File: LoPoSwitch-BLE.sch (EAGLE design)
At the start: 12 parts, among them Q1 2.5A/30V

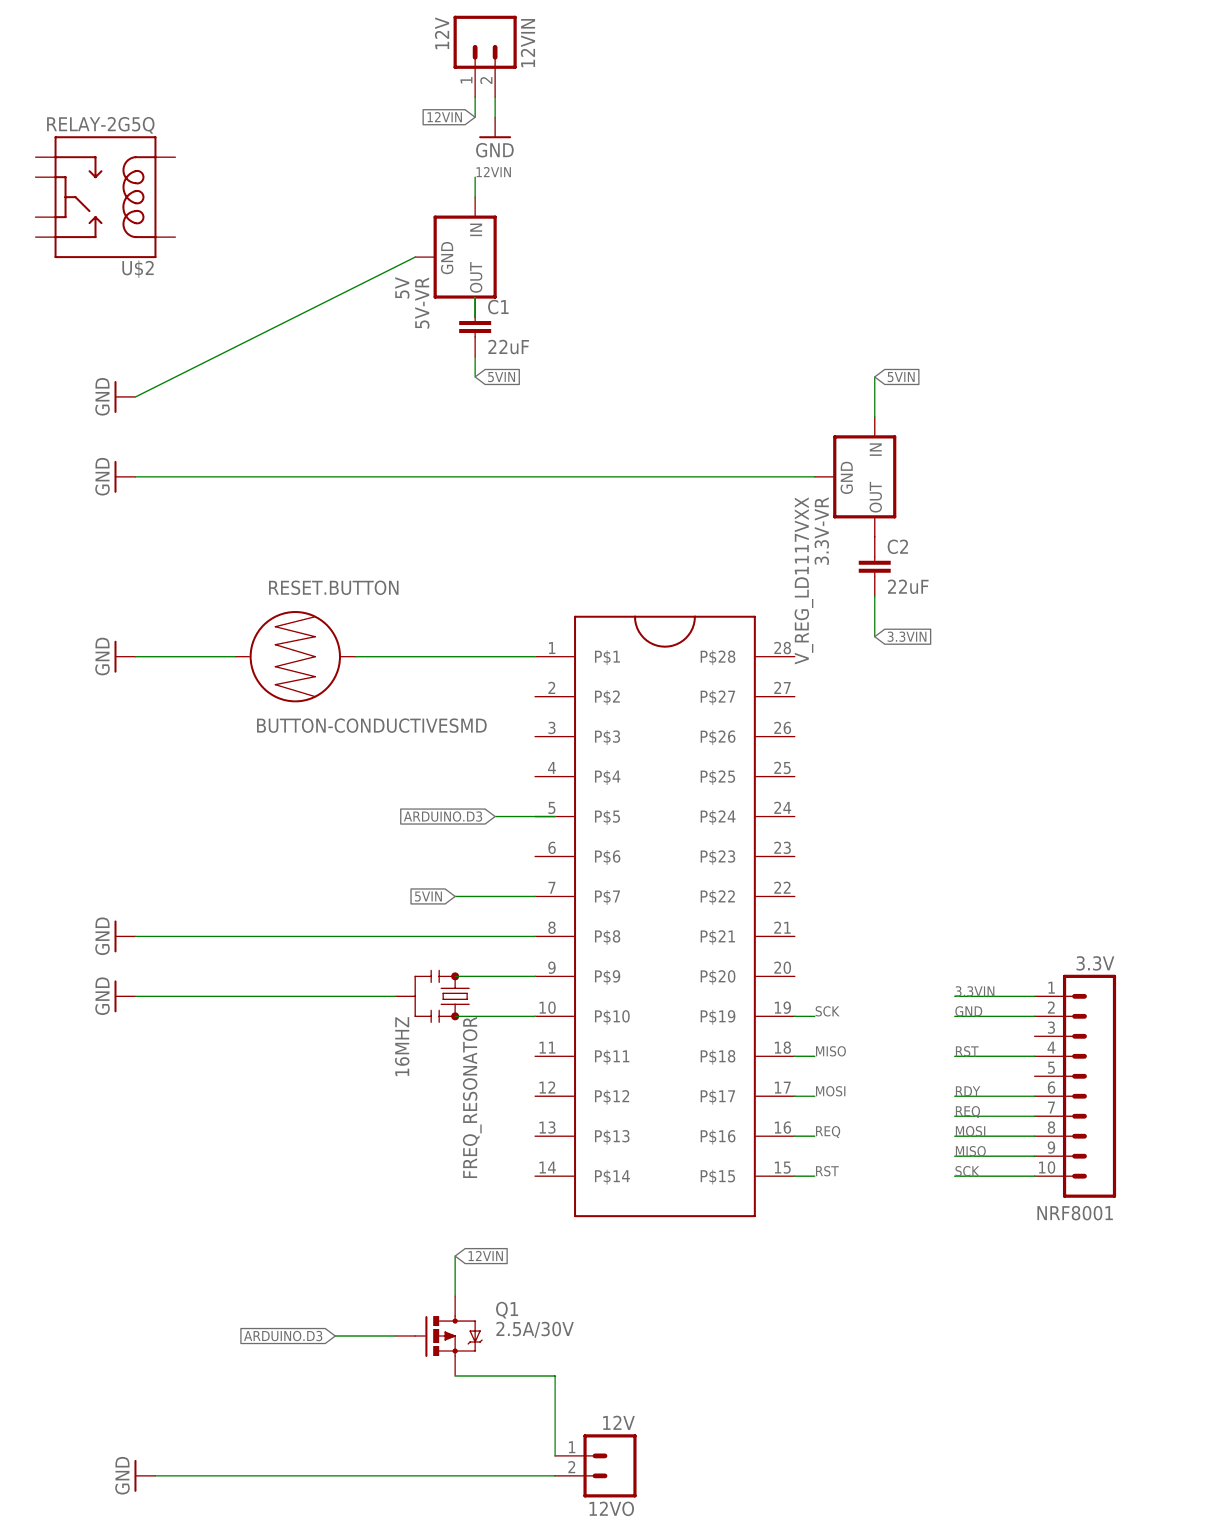
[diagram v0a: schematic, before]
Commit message: Restyle Board with SeedStudio Elements
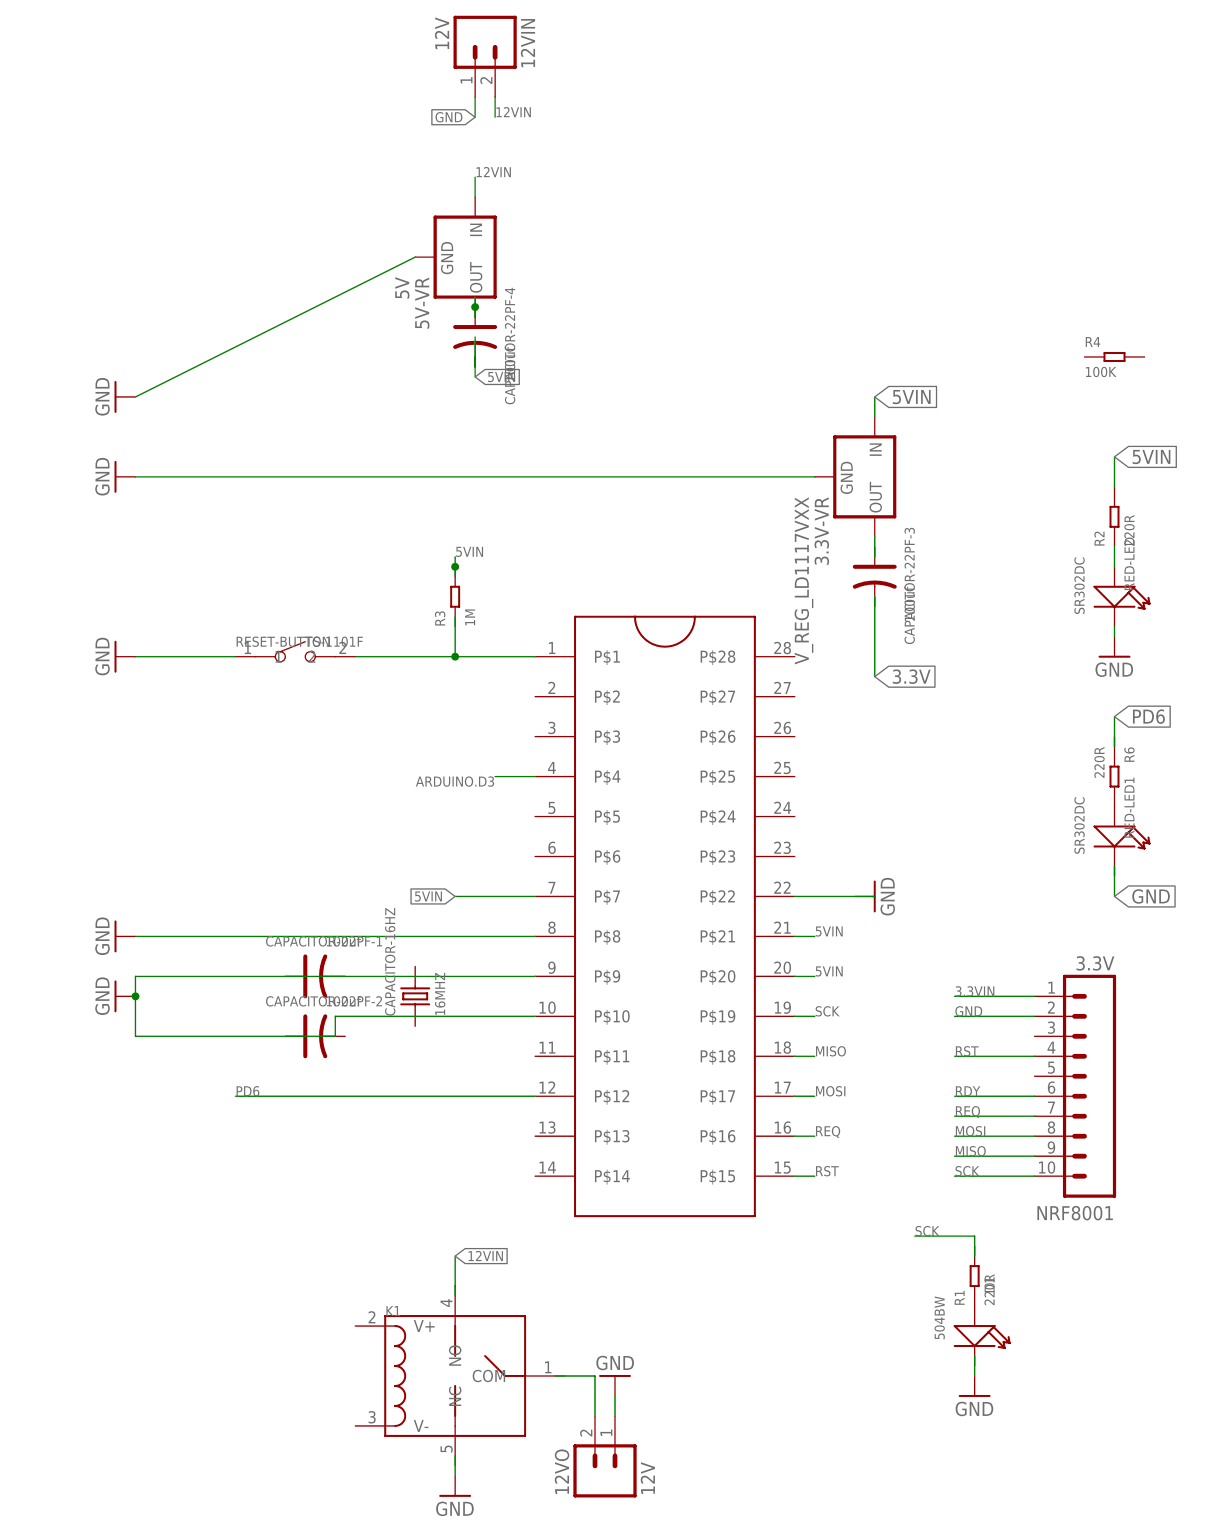
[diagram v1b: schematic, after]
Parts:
- removed C1, C2: 22uF, SparkFun-Capacitors:22UF-16V-20%-(1210)
- removed FREQ_RESONATOR: 16MHZ, SparkFun-FreqCtrl:RESONATOR16MHZ
- removed Q1: 2.5A/30V, SparkFun-DiscreteSemi:MOSFET-PCHANNELDMG2307L
- removed RESET.BUTTON: BUTTON-CONDUCTIVESMD, SparkFun-Electromechanical:BUTTON-CONDUCTIVESMD
- removed U$2: RELAY-2G5Q, SparkFun-Electromechanical:RELAY-2G5Q
- added CAPACITOR-16HZ: 16MHZ, Seeed-Crystal Oscillator:DIP-CRYSTAL-16MHZ-18PF-30PPM-50R(HC49US)
- added CAPACITOR-22PF-1, CAPACITOR-22PF-2, CAPACITOR-22PF-3, CAPACITOR-22PF-4: 100uf, Seeed-Capacitor:DIP-ALUMINUM-47UF-16V(D5-H7MM)
- added D1: 504BW, Seeed-LED:DIP-LED-BLUE-BLUE(2P-D5MM)
- added K1: (no value), Seeed-Relay:RELAY-HLS8L-DC5V-S-CHLS8L-DC5V-S-C
- added R1, R2, R6: 220R, Seeed-Resistor:DIP-RES-220R-5%-1/4W(PR-D2.3XL6.5MM)
- added R3: 1M, Seeed-Resistor:DIP-RES-1M-5%-1/4W(PR-D2.3XL6.5MM)
- added R4: 100K, Seeed-Resistor:DIP-RES-100K-5%-1/6W(PR-D1.8XL3.3MM)
- added RED-LED, RED-LED1: SR302DC, Seeed-LED:DIP-LED-RED-RED(2P-D3MM)
- added RESET-BUTTON: TS-1101F, Seeed-Switch:DIP-BUTTON(2P-6.0X3.0X4.3MM)-TS-1101F
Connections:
- removed net N$4: 12VO.1, Q1.S
- new net N$7: D1.+, R1.1
- new net N$8: R2.1, RED-LED.+
- new net N$9: ATMEGA328.P$22
- new net PD6: ATMEGA328.P$12, R6.1
- net 12VIN: now also 12VIN.2, K1.NO; no longer 12VIN.1, Q1.D
- net 3.3VIN: no longer C2.2
- net 5VIN: now also ATMEGA328.P$20, ATMEGA328.P$21, CAPACITOR-22PF-4.-, R2.2, R3.2; no longer C1.2
- net ARDUINO.D3: now also ATMEGA328.P$4; no longer Q1.G
- net GND: now also 12VIN.1, 12VO.1, ATMEGA328.P$10, ATMEGA328.P$9, RED-LED.-, RED-LED1.-, RESET-BUTTON.1; no longer 12VIN.2, 12VO.2, FREQ_RESONATOR.2, RESET.BUTTON.1
- net N$1: now also 12VO.2; no longer ATMEGA328.P$9, FREQ_RESONATOR.1
- net N$2: now also R6.2, RED-LED1.+; no longer ATMEGA328.P$10, FREQ_RESONATOR.3
- net N$3: now also RESET-BUTTON.2; no longer RESET.BUTTON.2
- net N$5: now also CAPACITOR-22PF-4.+; no longer C1.1
- net N$6: no longer C2.1
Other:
- moved on the sheet: 12VO
